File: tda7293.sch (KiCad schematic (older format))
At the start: 72 parts, among them J1 Screw_Terminal_01x04, J2 Conn_01x01_Male, J3 Screw_Terminal_01x02, J4 Conn_01x01_Male, J5 Conn_01x01_Male, J6 Conn_01x01_Male, J7 Conn_01x01_Male, J8 Conn_01x01_Male, J9 Conn_01x01_Male, Q1 BSS84, Q2 2N7002, U1 TDA7293, U2 TDA7293, U3 PC817, U4 MCP1792

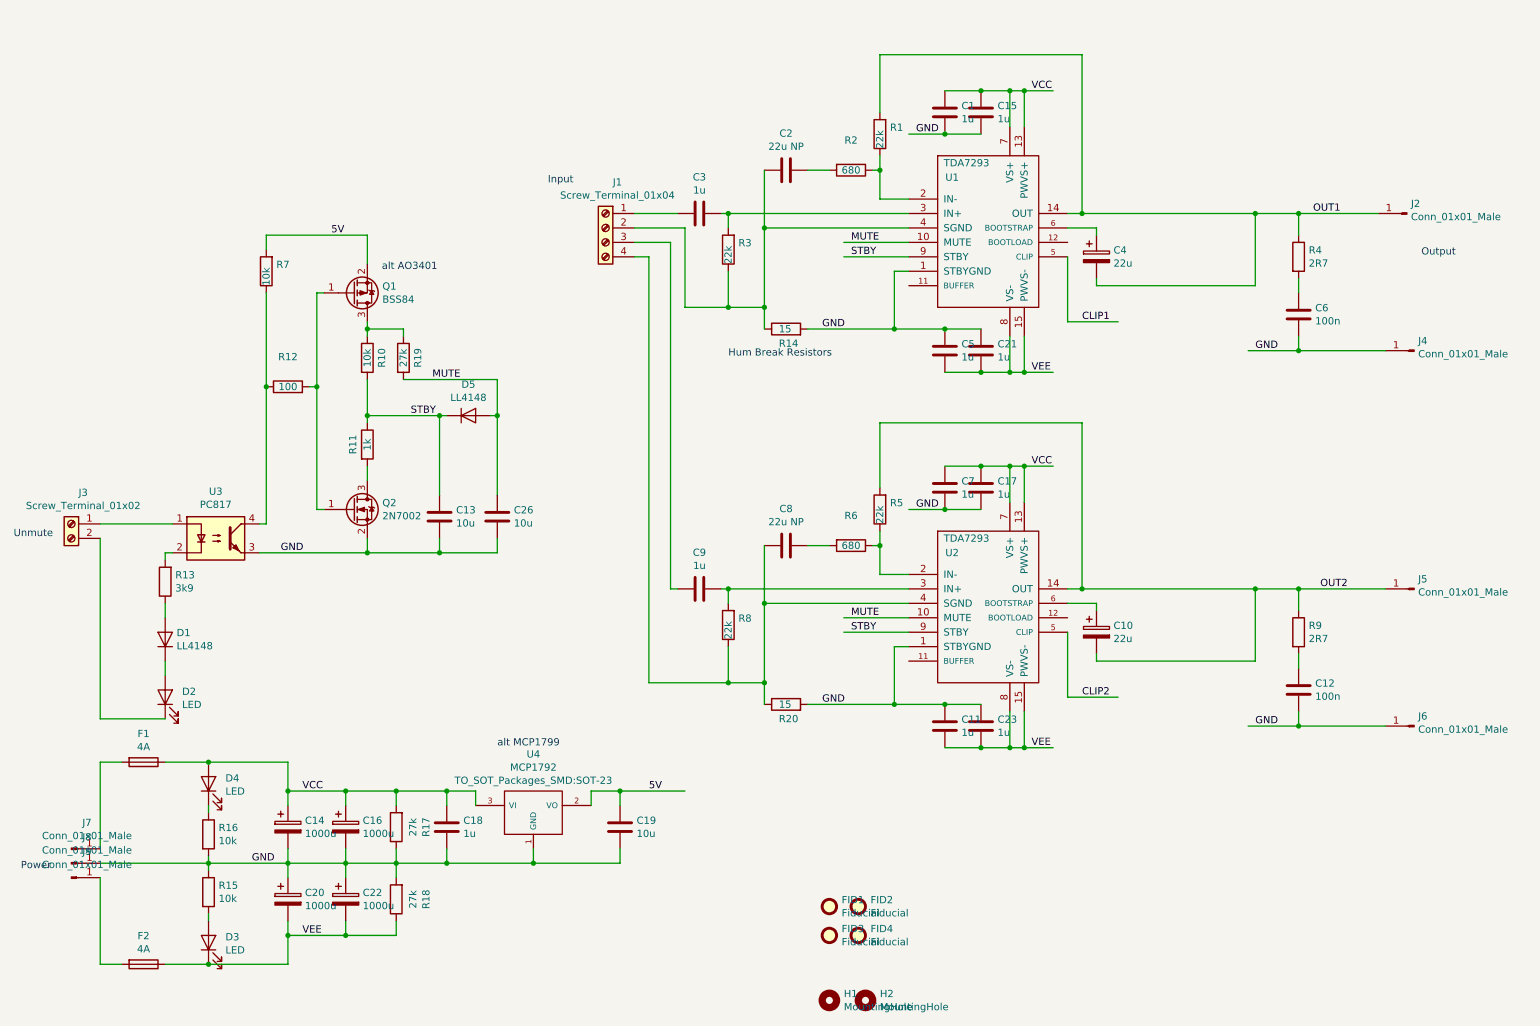
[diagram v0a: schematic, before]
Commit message: silk-screen updates, turd-polishing, plotted gerbers
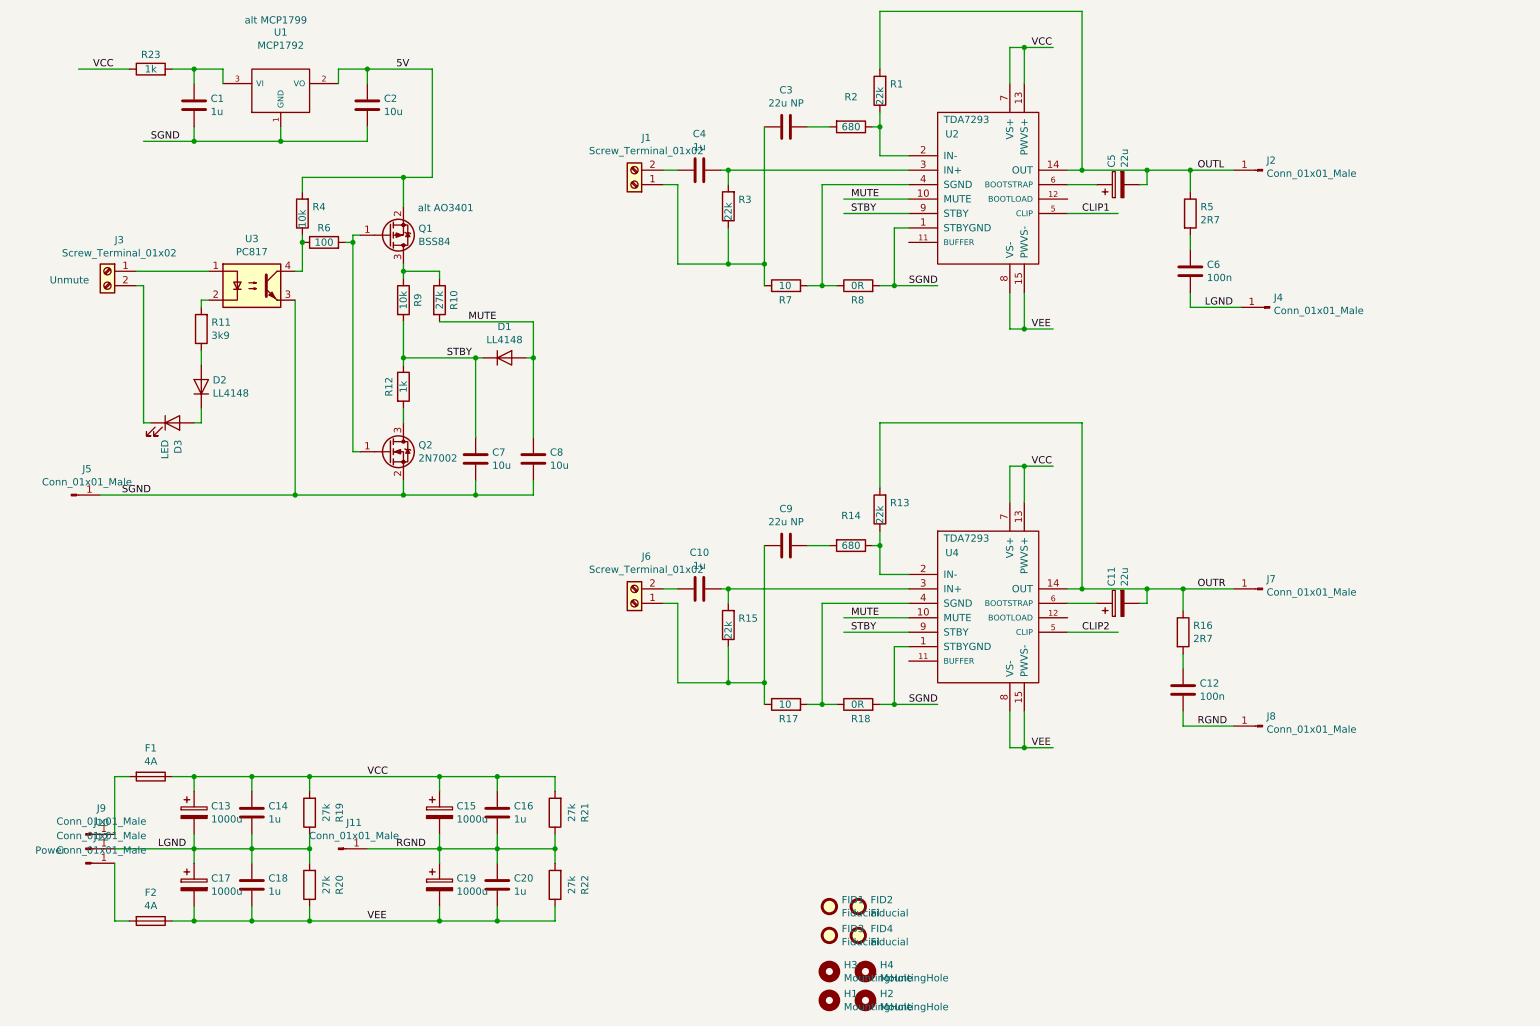
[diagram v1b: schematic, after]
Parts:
- removed C1, C11, C5, C7: 1u, Capacitors_SMD:C_0805, symbol Device:C
- removed D3, D4: LED, LEDs:LED_0805, symbol Device:LED
- removed J1: Screw_Terminal_01x04, Terminals_Phoenix:TerminalBlock_Phoenix_MPT-2.54mm_4pol, symbol Connector:Screw_Terminal_01x04
- removed R15, R16: 10k, Resistors_SMD:R_0805, symbol Device:R
- added H3, H4: MountingHole, Mounting_Holes:MountingHole_3.2mm_M3, symbol Mechanical:MountingHole
- added J1, J6: Screw_Terminal_01x02, Terminals_Phoenix:TerminalBlock_Phoenix_MPT-2.54mm_2pol, symbol Connector:Screw_Terminal_01x02
- added J11, J5: Conn_01x01_Male, power:FASTON250P_5.08mm_male_vertical, symbol Connector:Conn_01x01_Male
- added R18, R8: 0R, Resistors_SMD:R_0805, symbol Device:R
- added R21, R22: 27k, Resistors_SMD:R_0805, symbol Device:R
- added R23: 1k, Resistors_SMD:R_0805, symbol Device:R
- C11: renamed from C10; footprint Capacitors_ThroughHole:CP_Radial_D8.0mm_P3.50mm -> Capacitors_ThroughHole:CP_Radial_D6.3mm_P2.50mm
- C5: renamed from C4; footprint Capacitors_ThroughHole:CP_Radial_D8.0mm_P3.50mm -> Capacitors_ThroughHole:CP_Radial_D6.3mm_P2.50mm
- R17: renamed from R20; value 15 -> 10
- R7: renamed from R14; value 15 -> 10
- renumbered C18 to C1, C9 to C10, C14 to C13, C15 to C14, C16 to C15, C17 to C16, C20 to C17, C21 to C18, C22 to C19, C19 to C2, C23 to C20, C2 to C3, C3 to C4, C13 to C7, C26 to C8, C8 to C9, D5 to D1, D1 to D2, D2 to D3, J8 to J10, J9 to J12, J5 to J7, J6 to J8, J7 to J9, R19 to R10, R13 to R11, R11 to R12, R5 to R13, R6 to R14, R8 to R15, R9 to R16, R17 to R19, R18 to R20, R7 to R4, R4 to R5, R12 to R6, R10 to R9, U4 to U1, U1 to U2, U2 to U4
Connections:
- net labels added: LGND, OUTL, OUTR, RGND, SGND
- net labels removed: GND, OUT1, OUT2
- wire segments 204 -> 203
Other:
- note removed: "Hum Break Resistors"
- note removed: "Input"
- note removed: "Output"
- moved on the sheet: C1, C11, C12, C13, C14, C15, C16, C17, C18, C19, C2, C20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
